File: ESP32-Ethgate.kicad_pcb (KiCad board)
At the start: 2 copper layers, 76.2 x 38.1 mm, 52 parts, among them J1 USB_B_Micro, J2 HR911105A, Q1 UMH3N, U1 AMS1117-3.3, U2 ESP32-WROOM-32U, U3 CH340C, U4 50MHz, U5 LAN8720A, U6 USBLC6-2SC6

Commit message: more tweaks
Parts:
- R16, R20, R21, R22: value 49K9 -> 49R9
- R17, R18, R3, R7: value 1K -> 1K5

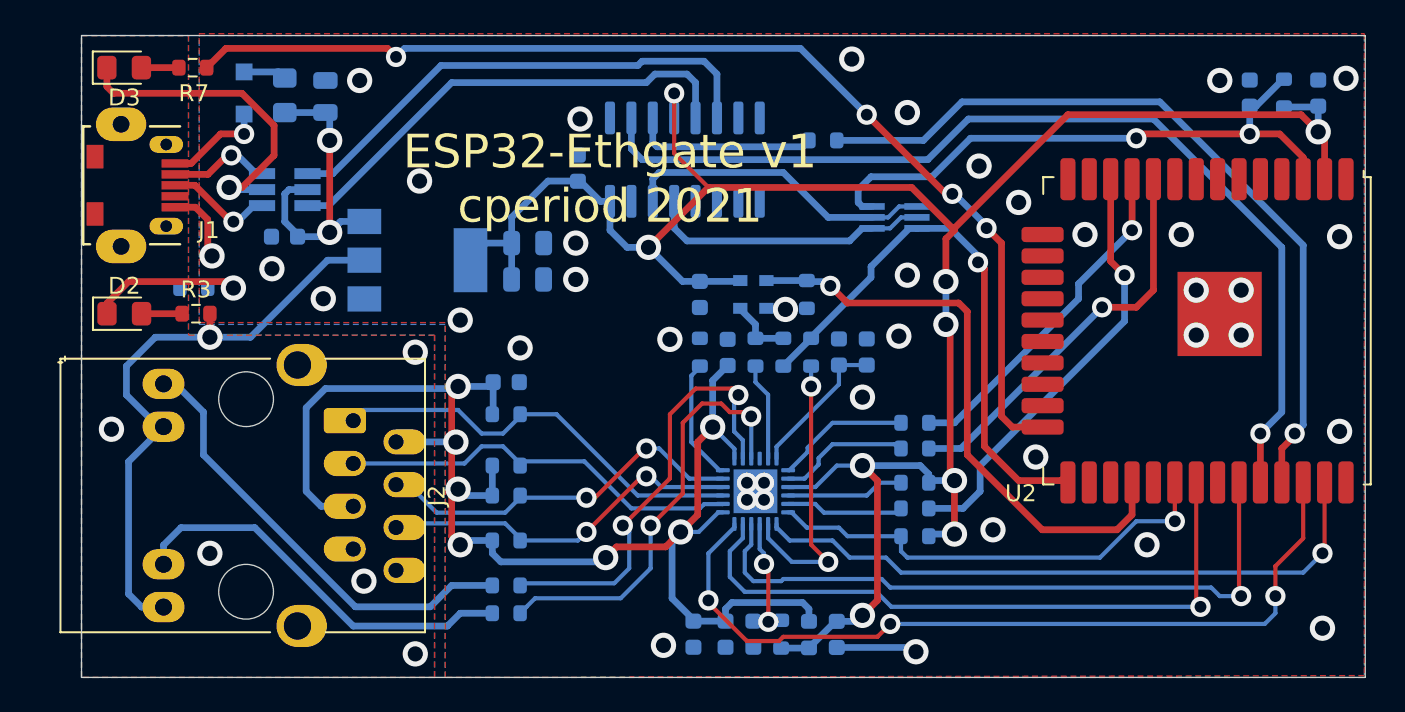
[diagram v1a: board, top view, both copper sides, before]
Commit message: better, but still not working.
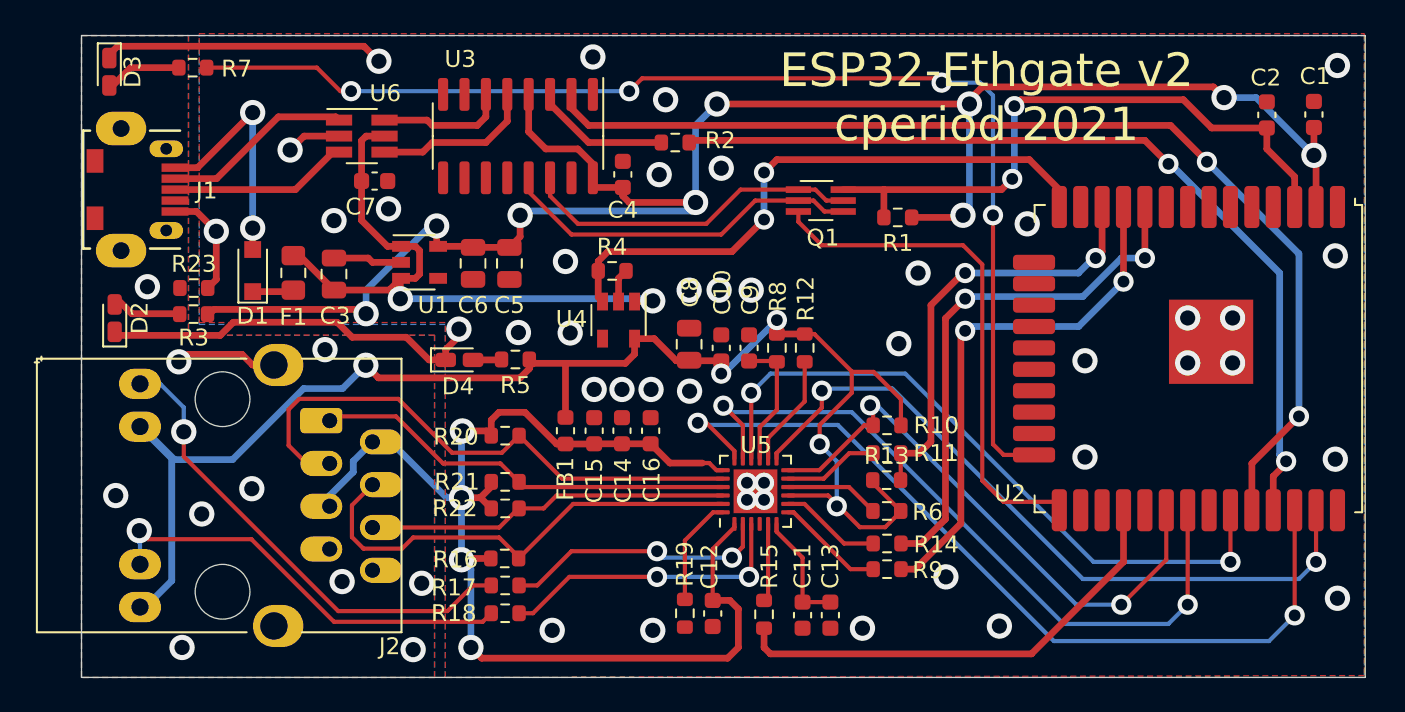
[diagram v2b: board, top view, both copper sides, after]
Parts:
- added D4: GREEN, LED_SMD:LED_0603_1608Metric_Castellated, F.Cu at (89.7, 80.2)
- added R4: 10K, Resistor_SMD:R_0603_1608Metric, F.Cu at (98.8, 74.9)
- C1, C10, C11, C12, C13, C14, C15, C16, C2, C3, C4, C5, C6, C7, C9, D1, F1, FB1, Q1, R1, R10, R11, R14, R15, R16, R17, R18, R19, R2, R20, R21, R22, R23, R8, R9, U3, U5, U6: moved to F.Cu
- C8: value 100n -> 22u; footprint Capacitor_SMD:C_0603_1608Metric -> Capacitor_SMD:C_0805_2012Metric; moved to F.Cu
- D2, D3: footprint LED_SMD:LED_0805_2012Metric_Pad1.15x1.40mm_HandSolder -> LED_SMD:LED_0603_1608Metric_Castellated
- R12: value 33R -> 10K; moved to F.Cu
- R13: value 33R -> 1K5; moved to F.Cu
- R5: value 10K -> 1K5; moved to F.Cu
- R6: value 10R -> 1K5; moved to F.Cu
- U1: value AMS1117-3.3 -> HT7233; footprint Package_TO_SOT_SMD:SOT-223-3_TabPin2 -> Package_TO_SOT_SMD:SOT-23-5; moved to F.Cu
- U4: value 50MHz -> HT7233; footprint Oscillator:Oscillator_SMD_Abracon_ASDMB-4Pin_2.5x2.0mm -> Package_TO_SOT_SMD:SOT-23-5; moved to F.Cu
- moved R1 24.1 mm to (115.8, 71.8), turned to 0 degrees
- moved FB1 18.9 mm to (96.0, 84.4), turned to 270 degrees
- moved C10 18.3 mm to (105.3, 79.5), turned to 90 degrees
- moved R5 17.7 mm to (93.1, 80.2), turned to 0 degrees
- moved C9 17.0 mm to (106.9, 79.5), turned to 90 degrees
- moved R8 17.0 mm to (108.6, 79.5), turned to 90 degrees
- moved C11 15.8 mm to (110.1, 95.4), turned to 270 degrees
- moved C13 15.8 mm to (111.8, 95.4), turned to 270 degrees
- moved R15 15.6 mm to (107.8, 95.3), turned to 90 degrees
- moved C12 15.5 mm to (104.8, 95.3), turned to 270 degrees
- moved R19 15.5 mm to (103.1, 95.2), turned to 90 degrees
- moved C15 14.4 mm to (97.7, 84.4), turned to 90 degrees
- moved C14 12.8 mm to (99.4, 84.4), turned to 90 degrees
- moved C3 10.6 mm to (82.3, 75.1)
- moved D1 10.6 mm to (77.5, 74.9), turned to 90 degrees
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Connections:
- C10 pad 1: +3V3 -> /+3V3_LAN
- C8 pad 1: +3V3 -> /+3V3_LAN
- FB1 pad 1: +3V3 -> /+3V3_LAN
- J2 pad 10: +3V3 -> /+3V3_LAN
- J2 pad 12: +3V3 -> /+3V3_LAN
- R10 pad 1: +3V3 -> /+3V3_LAN
- R12 pad 1: /IO0 -> /+3V3_LAN
- R13 pad 1: /IO0 -> /+3V3_LAN
- R13 pad 2: /CLOCK -> /CRS_DV
- R15 pad 1: /CLOCK -> /PHY_CLK
- R5 pad 1: /PHY_PWR -> Net-(D4-Pad2)
- R5 pad 2: GND -> /+3V3_LAN
- R6 pad 2: +3V3 -> /+3V3_LAN
- R8 pad 2: +3V3 -> /+3V3_LAN
- U1 pad 1: GND -> +5V
- U1 pad 2: +3V3 -> GND
- U2 pad 14: (no net) -> /PHY_POWER
- U2 pad 28: /PHY_PWR -> /PHY_CLK
- U4 pad 1: /PHY_PWR -> +5V
- U4 pad 3: /CLOCK -> /PHY_POWER
- U4 pad 4: +3V3 -> (no net)
- U5 pad 9: +3V3 -> /+3V3_LAN
- U6 pad 1: Net-(J1-Pad3) -> Net-(J1-Pad2)
- U6 pad 3: Net-(J1-Pad2) -> Net-(J1-Pad3)
- U6 pad 4: Net-(U3-Pad6) -> Net-(U3-Pad5)
- U6 pad 6: Net-(U3-Pad5) -> Net-(U3-Pad6)
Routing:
- net /+3V3_LAN: track 0.00 -> 92.6 mm, vias 0 -> 5
- net +3V3: track 167.7 -> 109.5 mm, vias 10 -> 9
- net /PHY_POWER: track 0.00 -> 36.3 mm, vias 0 -> 2
- net /PHY_PWR: track 35.6 -> 0.00 mm, vias 1 -> 0
- net /PHY_CLK: track 0.00 -> 28.5 mm
- net Net-(U3-Pad6): track 30.0 -> 7.69 mm
- net Net-(U3-Pad5): track 28.6 -> 9.63 mm
- net +5V: track 19.2 -> 37.9 mm
- net GND: track 37.4 -> 55.5 mm, vias 41 -> 42
- net +3.3VA: track 85.5 -> 73.6 mm, vias 7 -> 4
- net /RXD1: track 19.9 -> 30.8 mm, vias 1 -> 2
- net /LINKLED: track 26.3 -> 15.9 mm
- net Net-(R12-Pad2): track 17.0 -> 6.65 mm, vias 2 -> 0
- net /TXN: track 24.3 -> 33.9 mm
- net /ACTLED: track 26.2 -> 17.7 mm
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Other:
- board text added: "ESP32-Ethgate v2 cperiod 2021"
- board text removed: "ESP32-Ethgate v1 cperiod 2021"
